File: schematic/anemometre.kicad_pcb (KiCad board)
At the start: 2 copper layers, 69.2 x 72.4 mm, 38 parts, among them J1 Anemometre, J10 PWR_SEL, J2 AVR-ISP-6, J3 PORT_C_ADC, J4 PORT_B, J5 Opto_PB0, J6 TTL Serial, J7 INTs/Ts, J8 USB_B_Mini, J9 +5VDC, SW1 Reset, U1 ATmega328P-P, U2 4N25, U3 FT232RL, Y1 8MHz

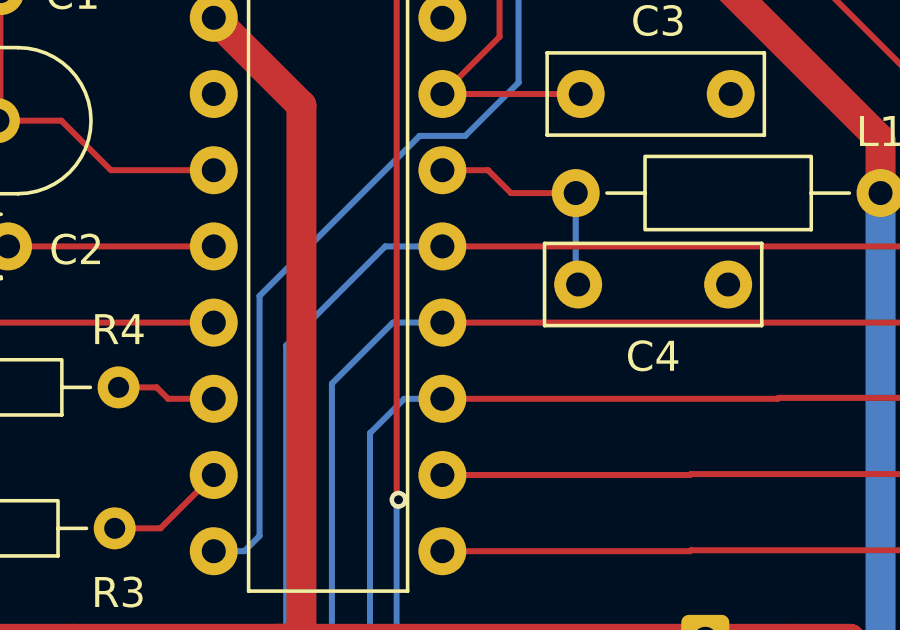
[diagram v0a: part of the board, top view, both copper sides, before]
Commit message: latest modifications and add raincounter sensor
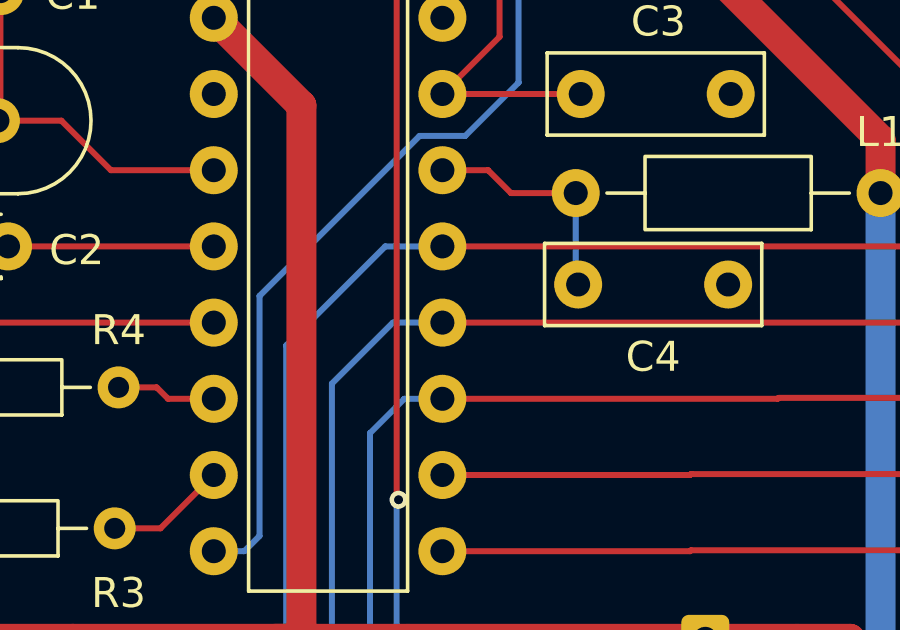
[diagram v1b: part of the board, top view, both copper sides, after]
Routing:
- net /MISO: track 61.9 -> 61.2 mm
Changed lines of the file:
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@@
-	)
-	(segment
-		(start 105.155 56.77)
-		(end 104.648 57.277)
-		(width 0.2)
-		(layer "F.Cu")
-		(net 12)
 	)
 	(segment
